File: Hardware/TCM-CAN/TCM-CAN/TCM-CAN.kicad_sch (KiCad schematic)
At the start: 4 parts, among them J2 Conn_01x27_Socket, J3 Conn_01x27_Socket, J4 Conn_02x20_Odd_Even, J5 Conn_01x06_Socket

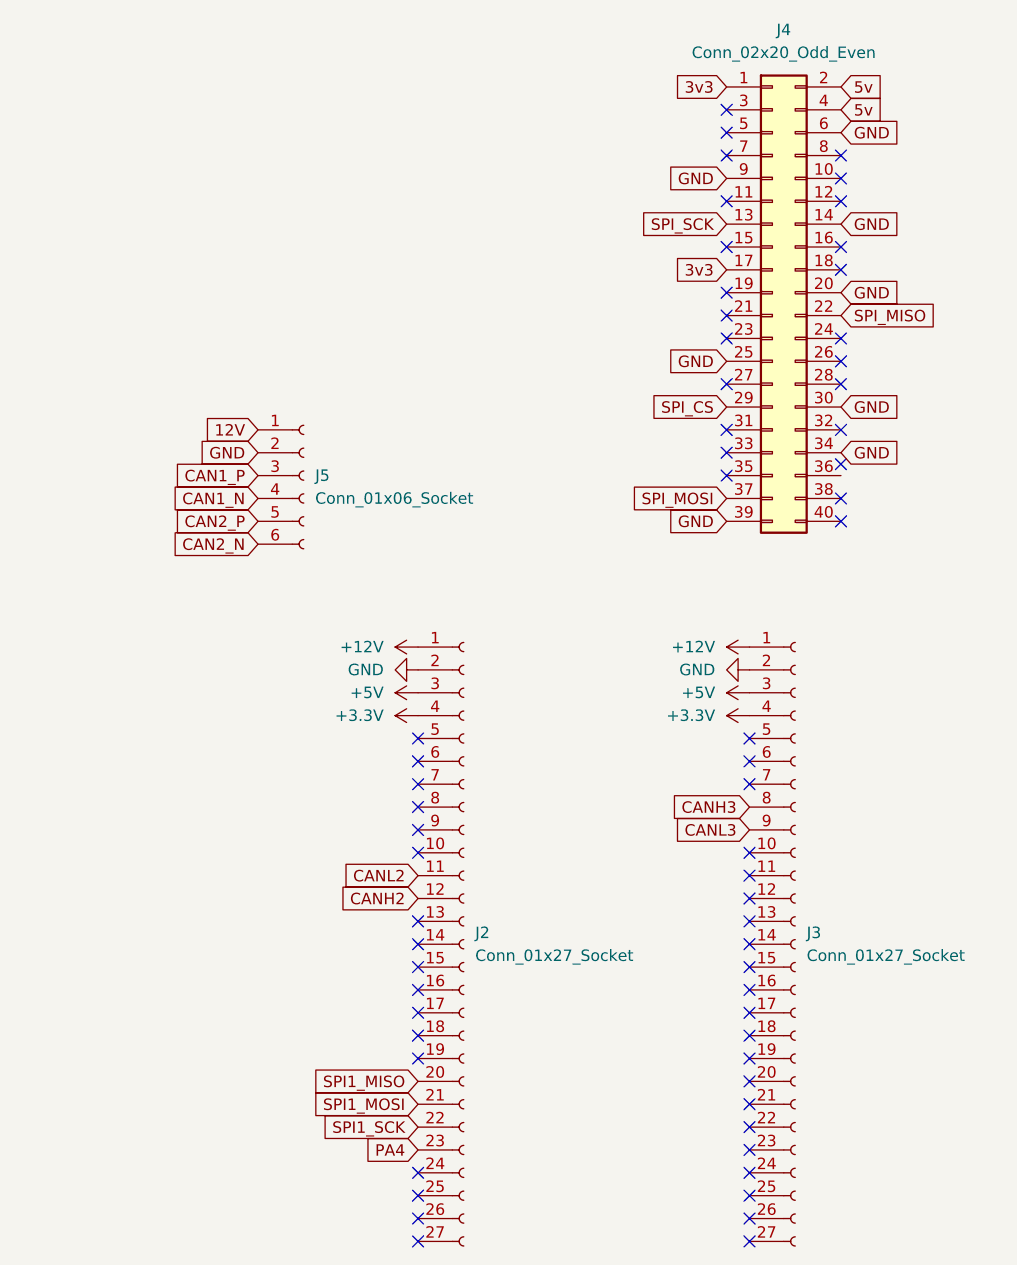
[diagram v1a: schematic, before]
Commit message: started work on the PCB for TCM-CAN
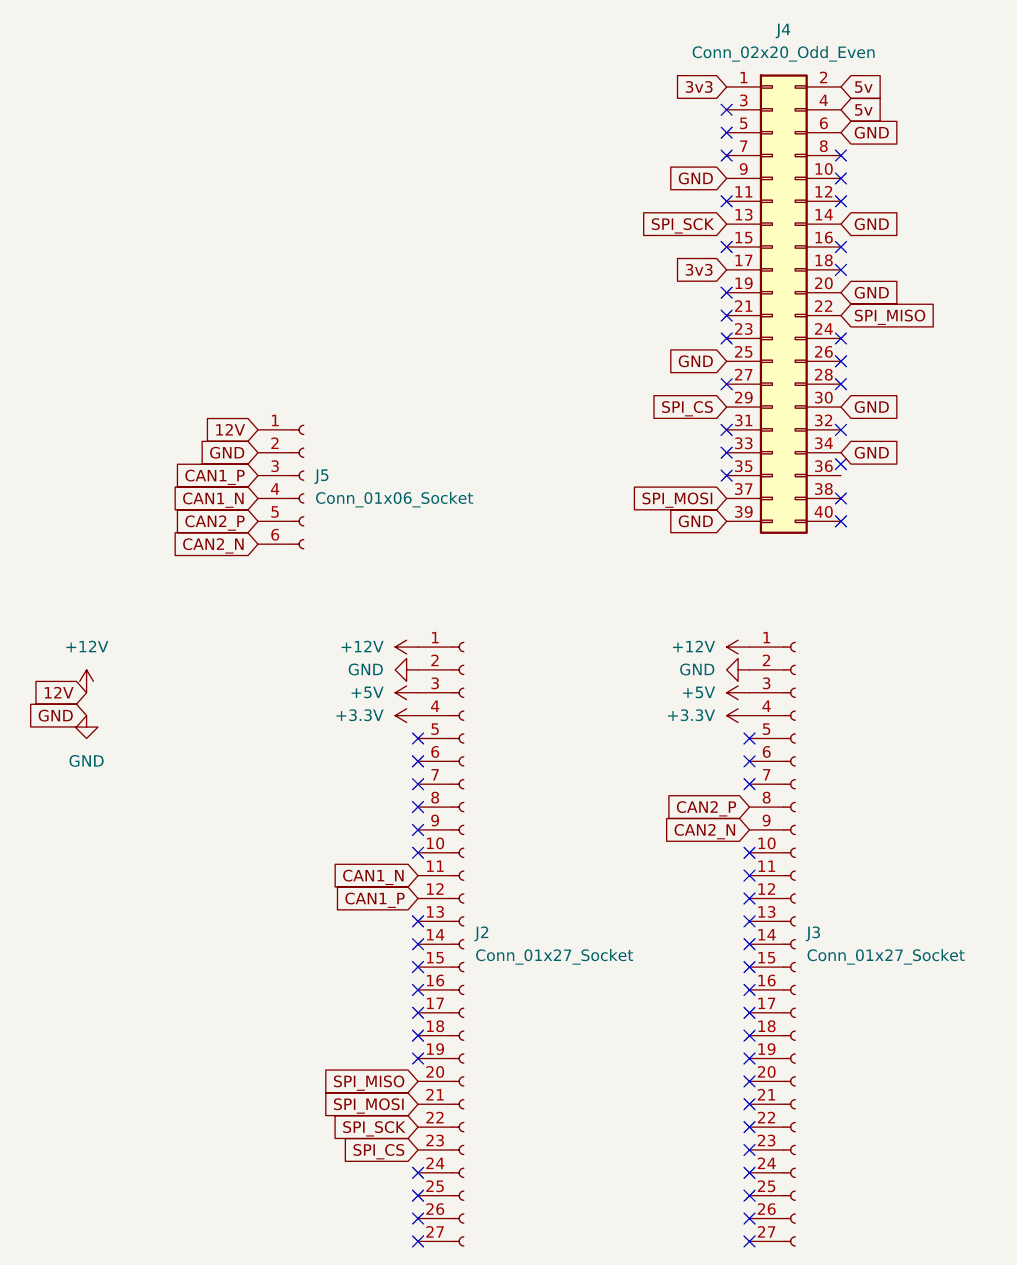
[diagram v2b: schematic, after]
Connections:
- net 12V is gone; now on net +12V: J5.1 (Pin_1)
- net CANH2 is gone; now on net CAN1_P: J2.12 (Pin_12)
- net CANH3 is gone; now on net CAN2_P: J3.8 (Pin_8)
- net CANL2 is gone; now on net CAN1_N: J2.11 (Pin_11)
- net CANL3 is gone; now on net CAN2_N: J3.9 (Pin_9)
- net PA4 is gone; now on net SPI_CS: J2.23 (Pin_23)
- net SPI1_MISO is gone; now on net SPI_MISO: J2.20 (Pin_20)
- net SPI1_MOSI is gone; now on net SPI_MOSI: J2.21 (Pin_21)
- net SPI1_SCK is gone; now on net SPI_SCK: J2.22 (Pin_22)
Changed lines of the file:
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@@
 			"AAAAAAAAAAAAAAAAAAAAAAAAAAAAAAAAAAAAAAAAAAAAAAAAAAAAAAAAAAAAAAAAAAAAAAAAAAAA"
 			"AAAAAAAAAAAAAAAAAAAAAAAAAAAAAAAAAAAAAAAAAAAAAAAAAAAAAAAAAAAAAAAAAAAAAAAAAAAA"
-			"AAAAAAAAAAAAAAAAAAAAAAAAAAAAAAAAAAAAAA=="
-		)
-	)
-	(global_label "SPI1_MISO"
+			"AAAAAAAAAAAAAAAAAAAAAAAAAAAAAAAAAAAAAES/KSSetSLGhBYknHemBjuztytAM6DSZ/kArfiO"
+			"5Qa5HT5Sswrq4DuQH2rppPQ55rUsgDFLSL0pa1IClpKKAHgnFOqOigCTOKaDTaB1oA811HQNLS8X"
+			"7frM82Q29ZbgKB0x/wDqqndXXhzTZFurKOJgzkMUBYyDI3DB/GtS/sfD6CdmAuJCyzM5LSbjkA8/"
+			"TtVZ9SsdQs5rLTbFkXymiEjRiNdx5A55H8XFc9r7Ht8zdnK7Qk/jASqEtLTaoYEF29Oeg/lWLqF/"
+			"eXxHnSswLcKBx+VX7PwhfRoEnnijK4wV5BHf34q9c2un6IodplkmwVbByTx6fWsGpv4mbylQjpTV"
+			"2cHcApdvnjkA561s6YxG1R03YI71nX8pnvJpcD945OP0q/p6BUX5s/MDj2q+h5ctZM3oQQmXGSet"
+			"XoCcqMZOecCq8CADgZyBxmr1pDhuTgZ6Z60FLRGgi4XqR6ZNTKuVyfwPaowjIMjnI47VLE20c4JN"
+			"UkQ2JJHlfnBJ7YqNFUd+vG01bOCMI4Df3c1G20HBAUnj5uM0xXIhtxngZ9aNueoAx/FTiAc7efao"
+			"9pJwHI9ulILgPc8dfl6ClzIx68j1xSqrLk8/N1zRj059dp4pgCktgAbW/u5GKeA38Q/DimHbuGWG"
+			"7GeTzipAwfHzZI7Yp3ExwDvjHI96cCqDGw59QaavTkH+VSKVC5JyPc0riIplWVMMuQezDNVo4BbY"
+			"VR8h9O1aW4bevB7Yo2LkHH6VDY7hDtdQrdanis4hljj1zio41VPu9fepwd6FSSMjtVJ3FZo4zW0S"
+			"O58yMBHJ3OR2Ungf59qitNQjjnVnPJ4J7GpfEkj3WpQ2cELYLfMwHVvT8MVK/haJ4l82do5RypVe"
+			"B6VLR0KS5dSa6utsiJbZxJztA6mrrsYVUSMFbb696qWVjLbgOwDSbT8+OgrLvXN7fxo8rgKclc43"
+			"VKbTuZytbQ14QEbzHc7s8AfwipmYtklnUe5rOS8H3SuD79anL7lO5g2O3WlcixcRlVcpj6tzT47n"
+			"5gWlB9qzBNJ8wViFA4G2rMEmM/Mc+m3pTTCyNTzw2QFYZ9qry5z8qsRRHO7tgfmxqWQ8EM5qiWis"
+			"211w2/H0rMuRGr/IrfjVmWZI8glmz2FUZ3zyqkUmNDWLMMZAA7U15fkwvQVGrnfggHFR3G/d049B"
+			"SBl6xk3yDBrr7IkxjPpXHWB2soA612NgP3QJ9K3pGUy8KdSAU6tzIMUYoooAKKKKACgdaKUdaAOD"
+			"g1Kytri4s7a2kmhGAqhcBHJbIOelM1aa9Zoo47RFt/MyJy2SOO6j8q0tTuRLG0JjtbXq26W4Xd0I"
+			"6Lk1mSahFfILVJ2uBgLss7Uken33/wAK53fZng=="
+		)
+	)
+	(global_label "SPI_MISO"
 		(shape input)
 		(at 180.34 130.81 180)
@@
 		)
 		(property "Intersheetrefs" "${INTERSHEET_REFS}"
-			(at 167.4972 130.81 0)
+			(at 168.7067 130.81 0)
 			(effects
 				(font
@@
 		)
 	)
-	(global_label "CANL3"
+	(global_label "12V"
+		(shape input)
+		(at 143.51 87.63 180)
+		(fields_autoplaced yes)
+		(effects
+			(font
+				(size 1.27 1.27)
+			)
+			(justify right)
+		)
+		(property "Intersheetrefs" "${INTERSHEET_REFS}"
+			(at 137.0172 87.63 0)
+			(effects
+				(font
+					(size 1.27 1.27)
+				)
+				(justify right)
+				(hide yes)
+			)
+		)
+	)
+	(global_label "CAN2_N"
 		(shape input)
 		(at 217.17 102.87 180)
@@
 		)
 		(property "Intersheetrefs" "${INTERSHEET_REFS}"
-			(at 208.2581 102.87 0)
-			(effects
-				(font
-					(size 1.27 1.27)
-				)
-				(justify right)
-				(hide yes)
-			)
-		)
-	)
-	(global_label "CANH2"
+			(at 206.9881 102.87 0)
+			(effects
+				(font
+					(size 1.27 1.27)
+				)
+				(justify right)
+				(hide yes)
+			)
+		)
+	)
+	(global_label "CAN1_P"
 		(shape input)
 		(at 180.34 110.49 180)
@@
 		)
 		(property "Intersheetrefs" "${INTERSHEET_REFS}"
-			(at 171.1257 110.49 0)
+			(at 170.2186 110.49 0)
 			(effects
 				(font
@@
 		)
 	)
-	(global_label "SPI1_MOSI"
+	(global_label "SPI_MOSI"
 		(shape input)
 		(at 180.34 133.35 180)
@@
 		)
 		(property "Intersheetrefs" "${INTERSHEET_REFS}"
-			(at 167.4972 133.35 0)
+			(at 168.7067 133.35 0)
 			(effects
 				(font
@@
 		)
 	)
-	(global_label "PA4"
+	(global_label "SPI_CS"
 		(shape input)
 		(at 180.34 138.43 180)
@@
 		)
 		(property "Intersheetrefs" "${INTERSHEET_REFS}"
-			(at 173.7867 138.43 0)
-			(effects
-				(font
-					(size 1.27 1.27)
-				)
-				(justify right)
-				(hide yes)
-			)
-		)
-	)
-	(global_label "SPI1_SCK"
+			(at 170.8234 138.43 0)
+			(effects
+				(font
+					(size 1.27 1.27)
+				)
+				(justify right)
+				(hide yes)
+			)
+		)
+	)
+	(global_label "SPI_SCK"
 		(shape input)
 		(at 180.34 135.89 180)
@@
 		)
 		(property "Intersheetrefs" "${INTERSHEET_REFS}"
-			(at 168.3439 135.89 0)
+			(at 169.5534 135.89 0)
 			(effects
 				(font
@@
 		)
 	)
-	(global_label "CANH3"
+	(global_label "CAN2_P"
 		(shape input)
 		(at 217.17 100.33 180)
@@
 		)
 		(property "Intersheetrefs" "${INTERSHEET_REFS}"
-			(at 207.9557 100.33 0)
+			(at 207.0486 100.33 0)
 			(effects
 				(font
@@
 		)
 	)
-	(global_label "CANL2"
+	(global_label "CAN1_N"
 		(shape input)
 		(at 180.34 107.95 180)
@@
 		)
 		(property "Intersheetrefs" "${INTERSHEET_REFS}"
-			(at 171.4281 107.95 0)
+			(at 170.1581 107.95 0)
 			(effects
 				(font
@@
 		(property "Intersheetrefs" "${INTERSHEET_REFS}"
 			(at 205.1134 55.88 0)
+			(effects
+				(font
+					(size 1.27 1.27)
+				)
+				(justify right)
+				(hide yes)
+			)
+		)
+	)
+	(global_label "GND"
+		(shape input)
+		(at 143.51 90.17 180)
+		(fields_autoplaced yes)
+		(effects
+			(font
+				(size 1.27 1.27)
+			)
+			(justify right)
+		)
+		(property "Intersheetrefs" "${INTERSHEET_REFS}"
+			(at 136.6543 90.17 0)
 			(effects
 				(font
@@
 				(path "/dce5d582-08ac-45e6-8e98-75b83df6efb2"
 					(reference "#PWR033")
+					(unit 1)
+				)
+			)
+		)
+	)
+	(symbol
+		(lib_id "power:GND")
+		(at 143.51 90.17 0)
+		(unit 1)
+		(exclude_from_sim no)
+		(in_bom yes)
+		(on_board yes)
+		(dnp no)
+		(fields_autoplaced yes)
+		(property "Reference" "#PWR02"
+			(at 143.51 96.52 0)
+			(effects
+				(font
+					(size 1.27 1.27)
+				)
+				(hide yes)
+			)
+		)
+		(property "Value" "GND"
+			(at 143.51 95.25 0)
+			(effects
+				(font
+					(size 1.27 1.27)
+				)
+			)
+		)
+		(property "Footprint" ""
+			(at 143.51 90.17 0)
+			(effects
+				(font
+					(size 1.27 1.27)
+				)
+				(hide yes)
+			)
+		)
+		(property "Datasheet" ""
+			(at 143.51 90.17 0)
+			(effects
+				(font
+					(size 1.27 1.27)
+				)
+				(hide yes)
+			)
+		)
+		(property "Description" "Power symbol creates a global label with name \"GND\" , ground"
+			(at 143.51 90.17 0)
+			(effects
+				(font
+					(size 1.27 1.27)
+				)
+				(hide yes)
+			)
+		)
+		(pin "1"
+		)
+		(instances
+			(project ""
+				(path "/dce5d582-08ac-45e6-8e98-75b83df6efb2"
+					(reference "#PWR02")
 					(unit 1)
 				)
@@
 					(unit 1)
 				)
+			)
+		)
+	)
+	(symbol
+		(lib_id "power:+12V")
+		(at 143.51 87.63 0)
+		(unit 1)
+		(exclude_from_sim no)
+		(in_bom yes)
+		(on_board yes)
+		(dnp no)
+		(fields_autoplaced yes)
+		(property "Reference" "#PWR01"
+			(at 143.51 91.44 0)
+			(effects
+				(font
+					(size 1.27 1.27)
+				)
+				(hide yes)
+			)
+		)
+		(property "Value" "+12V"
+			(at 143.51 82.55 0)
+			(effects
+				(font
+					(size 1.27 1.27)
+				)
+			)
+		)
+		(property "Footprint" ""
+			(at 143.51 87.63 0)
+			(effects
+				(font
+					(size 1.27 1.27)
+				)
+				(hide yes)
+			)
+		)
+		(property "Datasheet" ""
+			(at 143.51 87.63 0)
+			(effects
+				(font
+					(size 1.27 1.27)
+				)
+				(hide yes)
+			)
+		)
+		(property "Description" "Power symbol creates a global label with name \"+12V\""
+			(at 143.51 87.63 0)
+			(effects
+				(font
+					(size 1.27 1.27)
+				)
+				(hide yes)
+			)
+		)
+		(pin "1"
+		)
+		(instances
+			(project ""
+				(path "/dce5d582-08ac-45e6-8e98-75b83df6efb2"
+					(reference "#PWR01")
+					(unit 1)
+				)
